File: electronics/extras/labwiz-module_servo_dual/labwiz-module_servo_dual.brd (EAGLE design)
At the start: 16 x 33.2 mm, 8 parts, among them U1 NCP1402

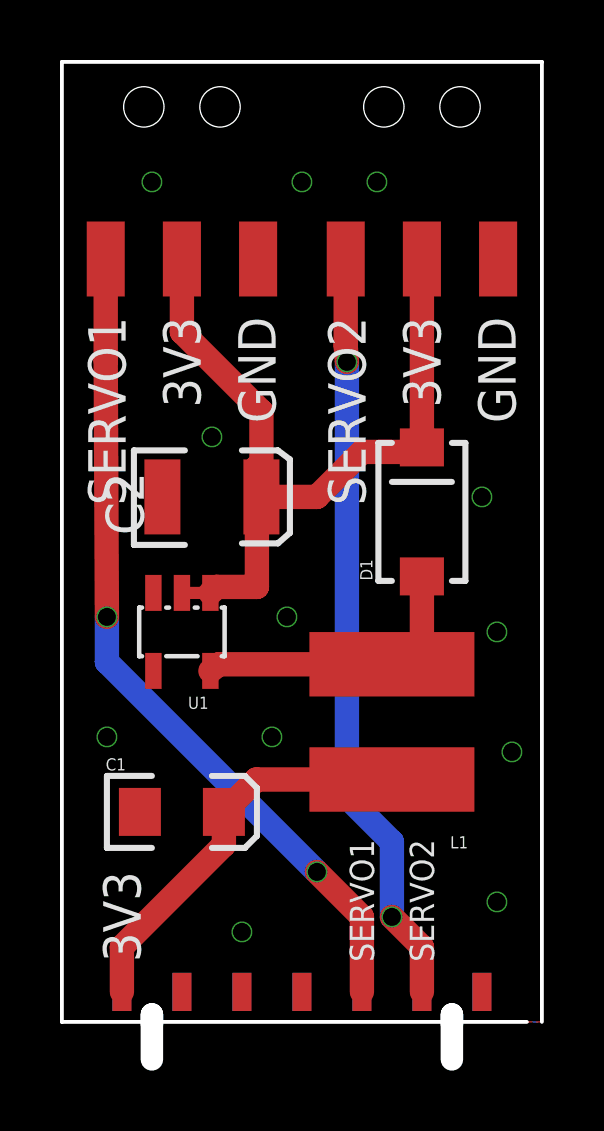
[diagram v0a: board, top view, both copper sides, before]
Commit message: Small changes. Not sure what.
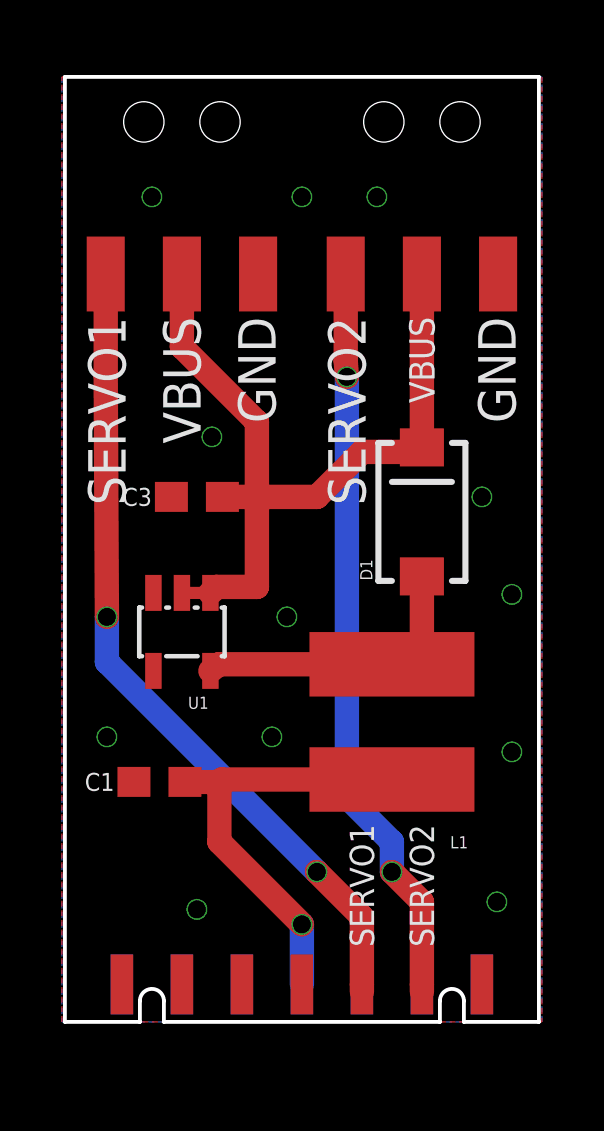
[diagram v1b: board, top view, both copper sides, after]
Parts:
- removed C2: 68uF, SparkFun:EIA3528
- added C3: 68uF, PaxInstruments-RCL:0603
- C1: device SparkFun:EIA3216 -> PaxInstruments-RCL:0603
- moved C1 1.25 mm to (3.25, 8.00)
- moved J1 0.50 mm to (4.00, 30.0)
- moved J2 0.50 mm to (12.0, 30.0)
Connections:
- removed net 3.3V: C1.A, L1.P$1, MODULE5.P$13
- removed net CANH: MODULE5.P$10
- removed net CANL: MODULE5.P$12
- removed net I2C_SCL: MODULE5.P$6
- removed net I2C_SDA: MODULE5.P$8
- removed net SPI_MISO: MODULE5.P$9
- removed net SPI_MOSI: MODULE5.P$11
- removed net SPI_SCK: MODULE5.P$7
- removed net USART_RX: MODULE5.P$4
- removed net USART_TX: MODULE5.P$2
- new net 3V3_A: MODULE5.P$13
- new net VBUS: C1.2, L1.P$1, MODULE5.P$8
- net 5V: now also C3.2; no longer C2.A
- net GND: now also C1.1, C3.1, MODULE5.P$2; no longer C1.C, C2.C
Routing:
- net VBUS: track 0.00 -> 14.8 mm, vias 0 -> 1
- net 3.3V: track 13.5 -> 0.00 mm
- net 5V: track 29.0 -> 27.3 mm
- net SERVO2: track 25.5 -> 25.0 mm
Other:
- board size 16 x 33.2 mm -> 15.8 x 31.5 mm
- board text added: "VBUS"
- board text removed: "3V3"
